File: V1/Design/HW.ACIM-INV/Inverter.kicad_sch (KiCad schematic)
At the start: 70 parts, among them J3 MOTOR, M1 560V/1.75kA, M2 560V/1.75kA, M3 560V/1.75kA, Q4 20V/1A, Q5 20V/1A, Q6 20V/1A, U1 IPM 600V/15A, U10 I=±10A, U3 ISEN 50mV/V, U7 I=±10A, U9 I=±10A

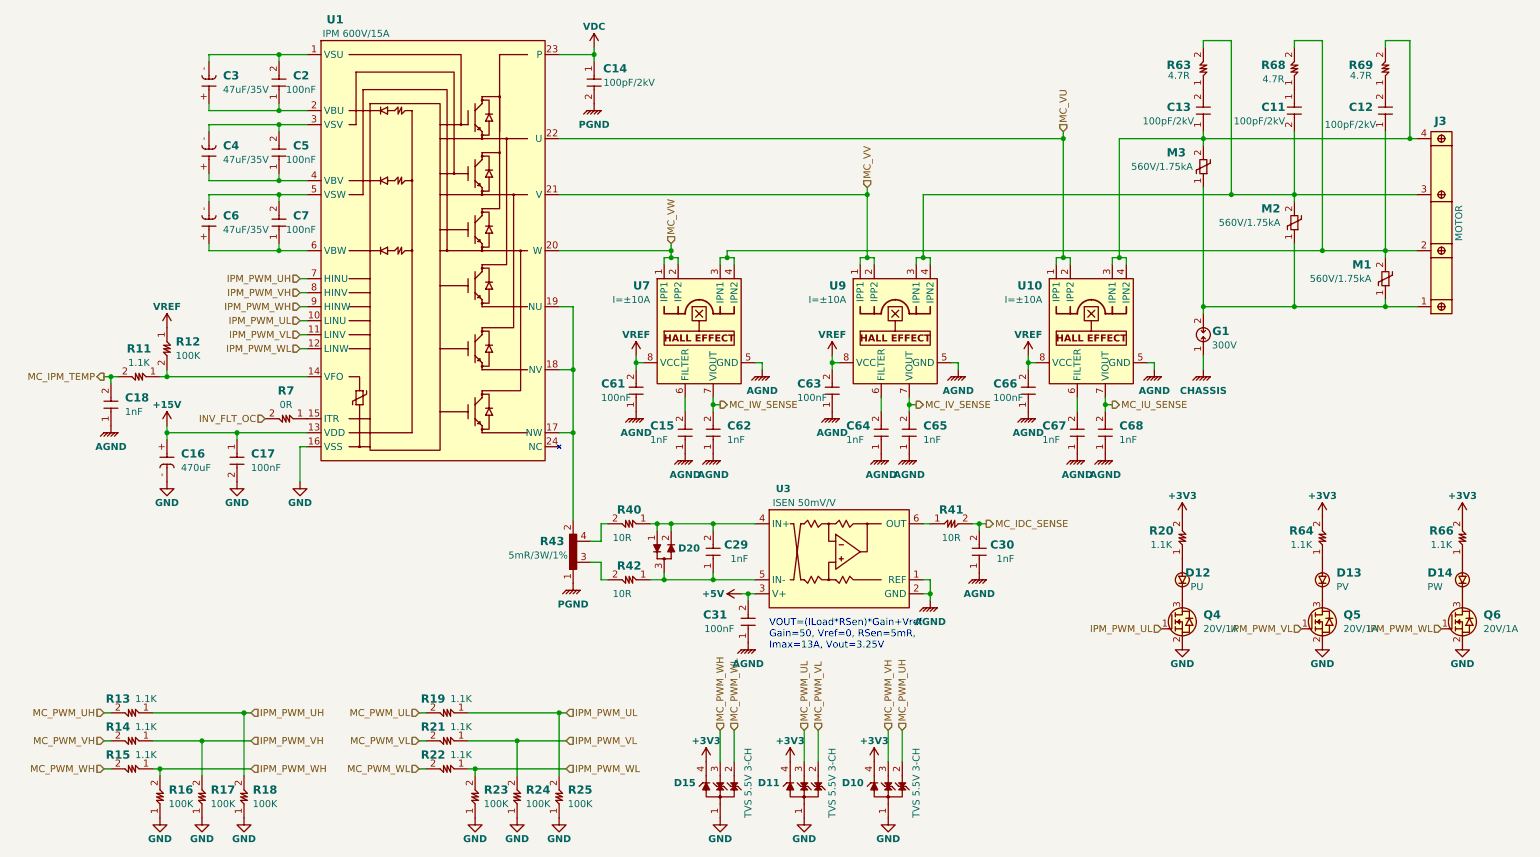
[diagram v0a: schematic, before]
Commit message: V1 schematic update 2
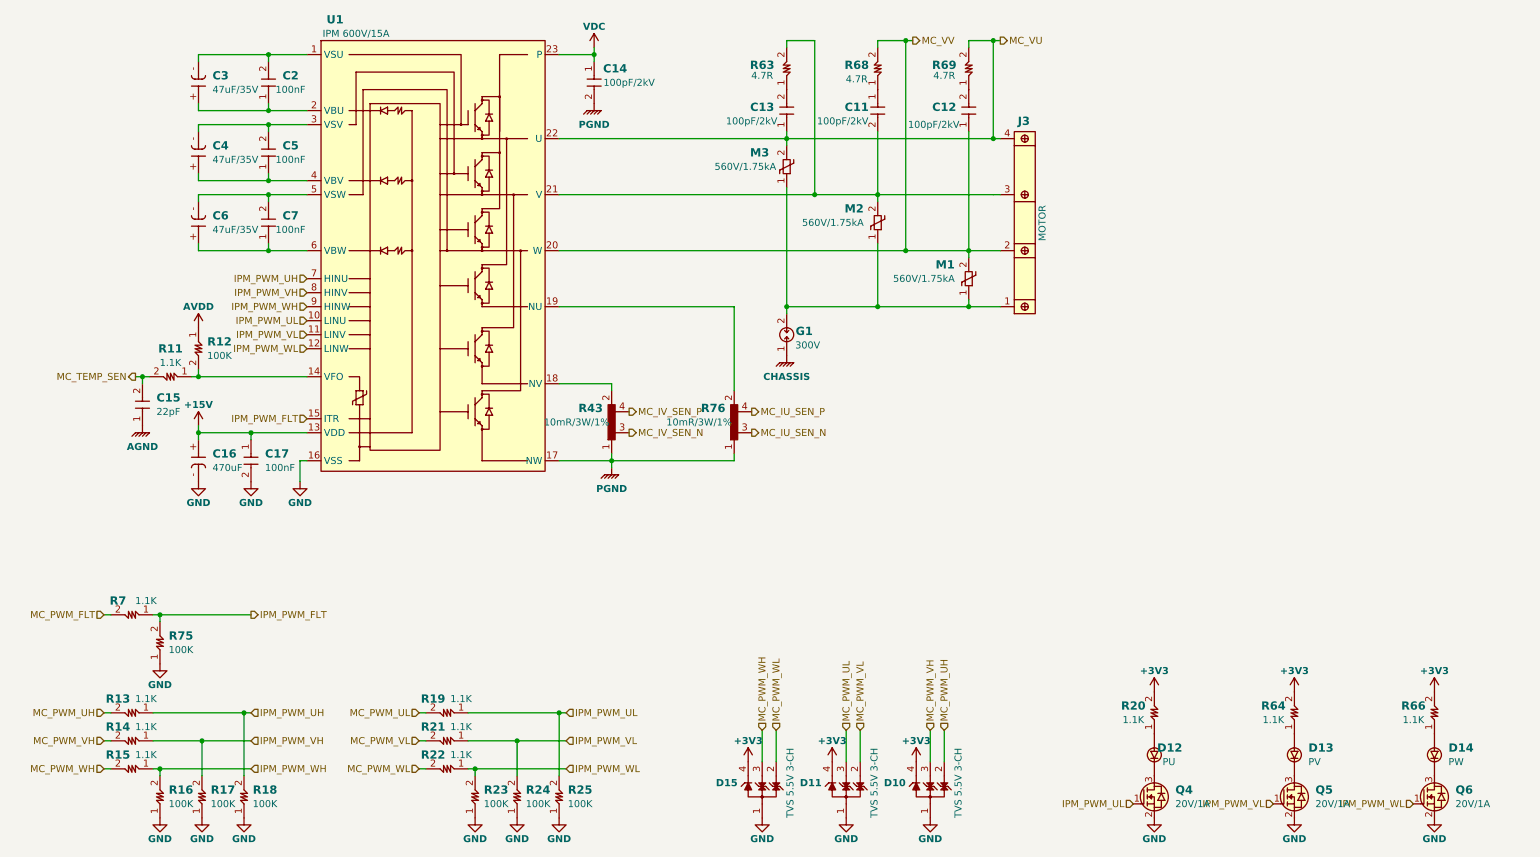
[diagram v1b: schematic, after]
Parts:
- removed C18, C29, C30, C62, C64, C65, C67, C68: 1nF, SAMPI:CAP0603, symbol SAMPI:CERCAP
- removed C31, C61, C63, C66: 100nF, SAMPI:CAP0603, symbol SAMPI:CERCAP
- removed D20: GP DIODE, SAMPI:SOT23, symbol SAMPI:DIODE_ARR1
- removed R40, R41, R42: 10R, SAMPI:RES0603, symbol SAMPI:RES
- removed U10, U7, U9: I=±10A, SAMPI:SOIC8_ALL, symbol SAMPI:ACS724
- removed U3: ISEN 50mV/V, SAMPI:SOT363, symbol SAMPI:ZXCT199Q
- added R75: 100K, SAMPI:RES0603, symbol SAMPI:RES
- added R76: 10mR/3W/1%, SAMPI:SHU2512, symbol SAMPI:SHUNT
- C15: value 1nF -> 22pF; MFT Samsung -> Walsin; MNP CL10B102KB8NNNC -> 0603N220J500CT; Unit Price 0.027 -> 0.012
- R43: value 5mR/3W/1% -> 10mR/3W/1%
- R7: value 0R -> 1.1K; MNP RC0603JR-070RL -> AC0603FR-071K1L; Unit Price 0.015 -> 0.021
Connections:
- net MC_IPM_TEMP is gone; now on net MC_TEMP_SEN: R11.2
- net MC_VW is gone; now on net MC_VV: U1.20 (W)
- net GND: now also R75.1
- net MC_VU: now also C13.1, J3.4, M3.2, R69.2
- net MC_VV: now also C12.1, J3.2, M1.2, R68.2; no longer U1.21 (V)
- net PGND: now also U1.17 (NW), R76.1
- net at C11.2, J3.3, M2.2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: now also U1.21 (V)
- net MC_IV_SEN_P: now reaches R43.4
- net IPM_PWM_FLT: now reaches R7.1, U1.15 (ITR)
- net IPM_PWM_FLT: now also R75.2
- net at R43.2, U1.18 (NV): no longer U1.17 (NW), U1.19 (NU)
- net MC_IV_SEN_N: now reaches R43.3
- net MC_TEMP_SEN: now reaches C15.2
- net INV_FLT_OC renamed MC_PWM_FLT
- net VREF renamed AVDD
- new net: R76.2, U1.19 (NU)
- new net MC_IU_SEN_N: R76.3
- new net MC_IU_SEN_P: R76.4
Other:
- note removed: "VOUT=(ILoad*RSen)*Gain+Vref Gain=50, Vref=0, RSen=5mR, Imax=13A, Vout=3.25V"
- moved on the sheet: C11, C12, C13, C16, C17, C2, C3, C4, C5, C6, C7, D10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
